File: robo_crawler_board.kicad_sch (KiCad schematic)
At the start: 14 parts, among them J1 Screw_Terminal_01x02, J2 Screw_Terminal_01x02, J3 Screw_Terminal_01x02, U2 DRV8262DDVR, U4 DRV8871DDA, U5 DRV8871DDA

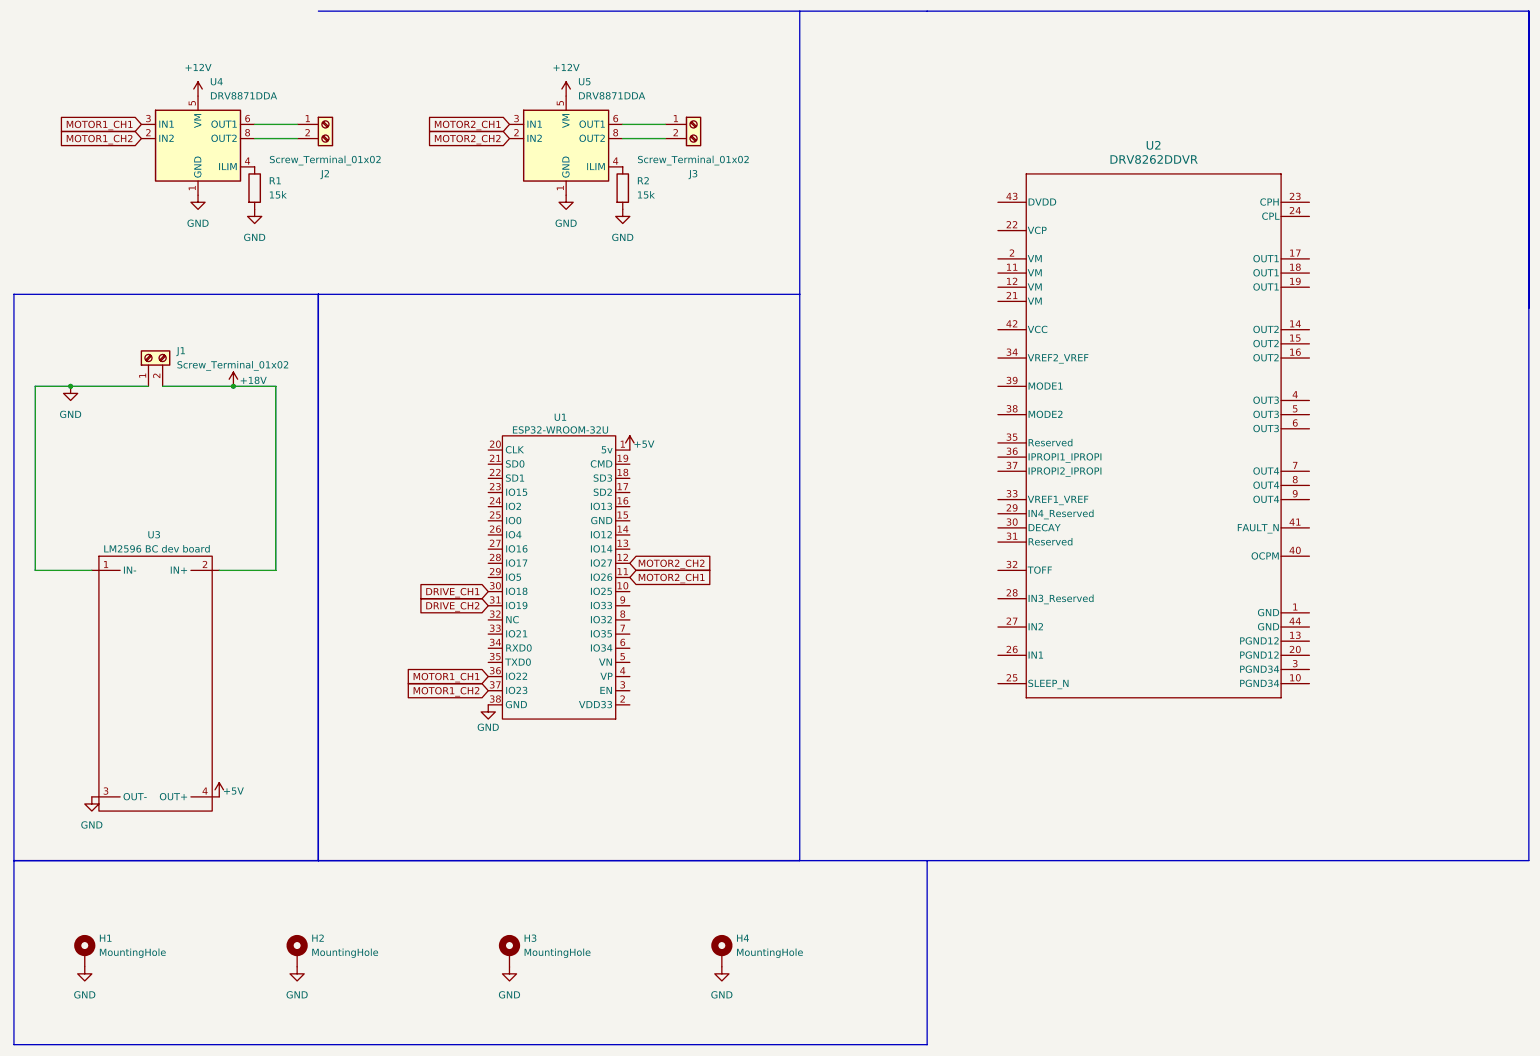
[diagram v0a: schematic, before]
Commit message: rev3 pcb done except ground planes
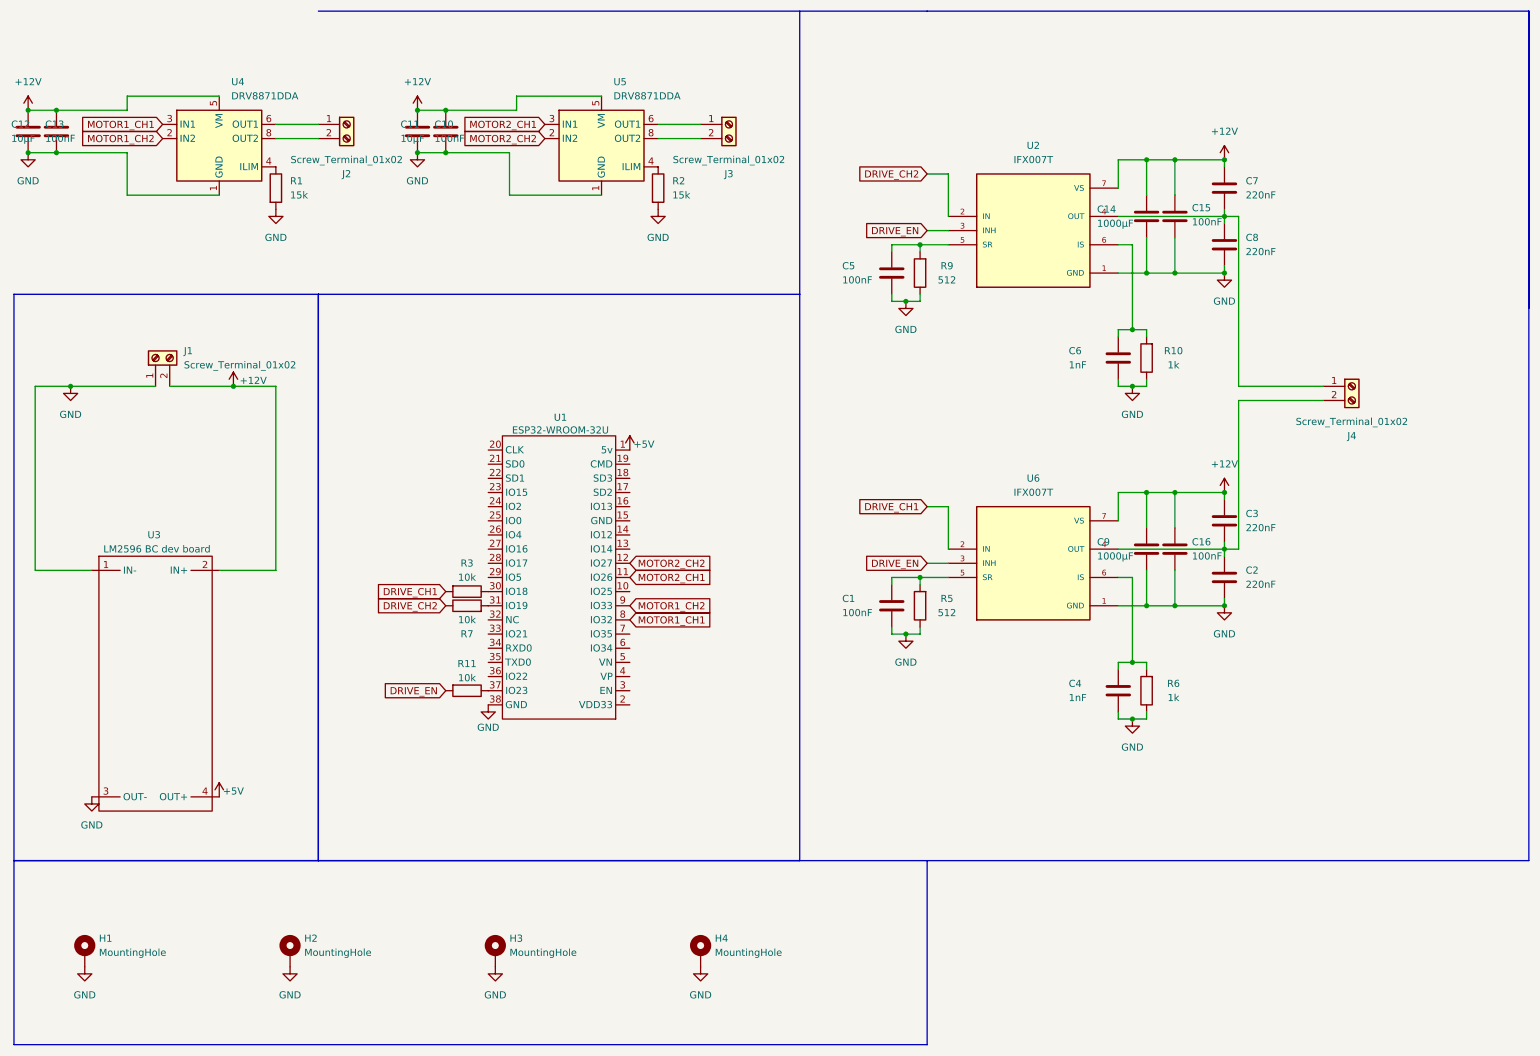
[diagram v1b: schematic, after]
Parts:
- removed U2: DRV8262DDVR, DDV0044E-IPC_A, symbol DRV8262DDVR:DRV8262DDVR
- added C1, C10, C13, C15, C16, C5: 100nF, Capacitor_SMD:C_0805_2012Metric, symbol Device:C
- added C11, C12: 10µF, Capacitor_SMD:C_0805_2012Metric, symbol Device:C
- added C14, C9: 1000µF, Capacitor_THT:CP_Radial_D10.0mm_P5.00mm, symbol Device:C
- added C2, C3, C7, C8: 220nF, Capacitor_SMD:C_0805_2012Metric, symbol Device:C
- added C4, C6: 1nF, Capacitor_SMD:C_0805_2012Metric, symbol Device:C
- added J4: Screw_Terminal_01x02, TerminalBlock:TerminalBlock_bornier-2_P5.08mm, symbol Connector:Screw_Terminal_01x02
- added R10, R6: 1k, Resistor_SMD:R_0805_2012Metric, symbol Device:R
- added R11, R3, R7: 10k, Resistor_SMD:R_0805_2012Metric, symbol Device:R
- added R5, R9: 512, Resistor_SMD:R_0805_2012Metric, symbol Device:R
- added U2, U6: IFX007T, ifx007t half-bridge:TO127P1500X440-8N, symbol ifx007t half-bridge:IFX007T
- R1, R2: LCSC Part Number (none) -> C17475
- U4, U5: LCSC Part Number (none) -> C1556867
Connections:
- net +18V is gone; now on net +12V: J1.2 (Pin_2), U3.2 (IN+)
- net +12V: now also C10.1, C11.1, C12.1, C13.1, C14.1, C15.1, C16.1, C3.1, C7.1, C9.1, U2.7 (VS), U6.7 (VS)
- net DRIVE_CH1: now also R3.2, U6.2 (IN); no longer U1.30 (IO18)
- net DRIVE_CH2: now also R7.1, U2.2 (IN); no longer U1.31 (IO19)
- net GND: now also C1.2, C10.2, C11.2, C12.2, C13.2, C14.2, C15.2, C16.2, C2.2, C4.2, C5.2, C6.2, C8.2, C9.2, R10.1, R5.1, R6.1, R9.1, U2.1 (GND), U6.1 (GND)
- net MOTOR1_CH1: now also U1.8 (IO32); no longer U1.36 (IO22)
- net MOTOR1_CH2: now also U1.9 (IO33); no longer U1.37 (IO23)
- new net: C6.1, R10.2, U2.6 (IS)
- new net: R3.1, U1.30 (IO18)
- new net: R7.2, U1.31 (IO19)
- new net: R11.1, U1.37 (IO23)
- new net: C4.1, R6.2, U6.6 (IS)
- new net: C7.2, C8.1, J4.1 (Pin_1), U2.4 (OUT), U2.8 (OUT)
- new net: C1.1, R5.2, U6.5 (SR)
- new net: C5.1, R9.2, U2.5 (SR)
- new net: C2.1, C3.2, J4.2 (Pin_2), U6.4 (OUT), U6.8 (OUT)
- new net DRIVE_EN: R11.2, U2.3 (INH), U6.3 (INH)
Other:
- moved on the sheet: H2, H3, H4, J1, J2, J3, R1, R2, U4, U5
